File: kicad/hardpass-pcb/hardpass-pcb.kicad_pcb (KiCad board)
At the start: 2 copper layers, 30 x 65 mm, 37 parts, among them P1 Pi_Zero, P2 OLED_I2C, SW1 1, SW10 C/UP, SW11 0/OK, SW12 OK/DN, SW2 2, SW3 3, SW4 4, SW5 5, SW6 6, SW7 7, SW8 8, SW9 9, U2 ESP-12E

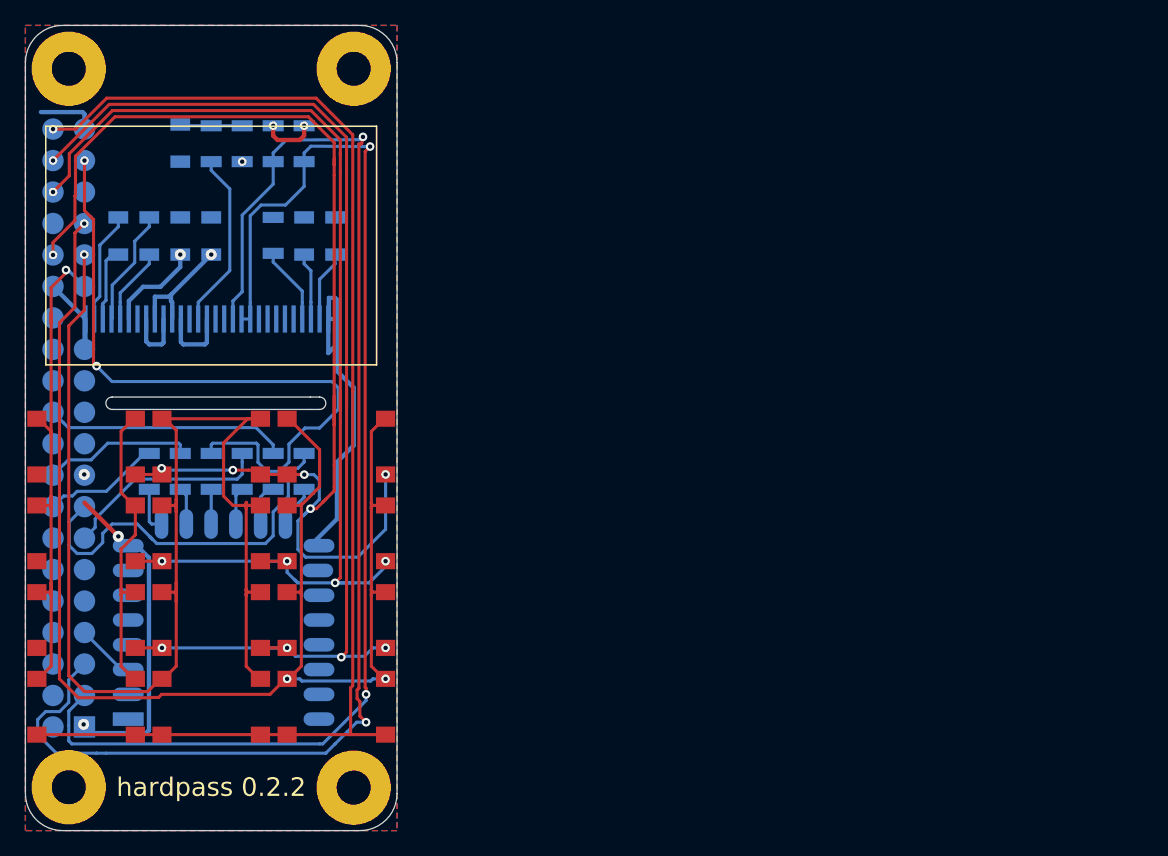
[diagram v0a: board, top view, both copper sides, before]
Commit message: routed 2nd board
not finished, but a start
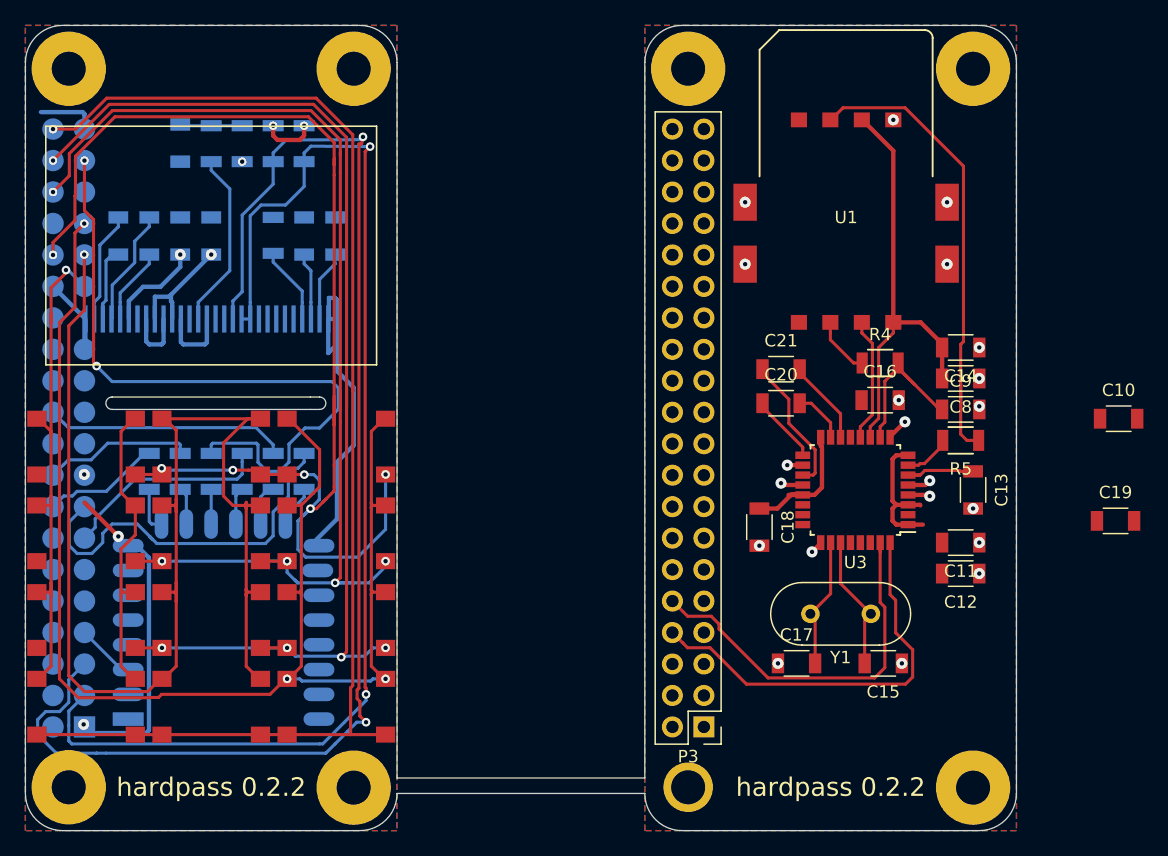
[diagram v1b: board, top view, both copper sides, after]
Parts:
- added C10: 100pF, Capacitors_SMD:C_1206, F.Cu at (88.2, 31.8)
- added C11: 10µF, Capacitors_SMD:C_1206, F.Cu at (75.5, 41.8)
- added C12: 100nF, Capacitors_SMD:C_1206, F.Cu at (75.5, 44.2)
- added C13: 22nF, Capacitors_SMD:C_1206, F.Cu at (76.5, 37.5)
- added C14: 100pF, Capacitors_SMD:C_1206, F.Cu at (75.5, 26.0)
- added C15: 22pF, Capacitors_SMD:C_1206, F.Cu at (69.2, 51.5)
- added C16: 220nF, Capacitors_SMD:C_1206, F.Cu at (69.0, 30.2)
- added C17: 22pF, Capacitors_SMD:C_1206, F.Cu at (62.2, 51.5)
- added C18: 100nF, Capacitors_SMD:C_1206, F.Cu at (59.2, 40.5)
- added C19: 10µF, Capacitors_SMD:C_1206, F.Cu at (88.0, 40.0)
- added C20: 220nF, Capacitors_SMD:C_1206, F.Cu at (61.0, 30.5)
- added C21: 220nF, Capacitors_SMD:C_1206, F.Cu at (61.0, 27.8)
- added C8: 220nF, Capacitors_SMD:C_1206, F.Cu at (75.5, 28.5)
- added C9: 33pF, Capacitors_SMD:C_1206, F.Cu at (75.5, 31.0)
- added P3: Pi_Zero, hardpass:Pin_Header_Straight_2x20_Pitch2.54mm_centered, F.Cu at (53.5, 32.5)
- added R4: 100, Resistors_SMD:R_1206, F.Cu at (69.0, 27.2)
- added R5: 180, Resistors_SMD:R_1206, F.Cu at (75.5, 33.5)
- added REF**: 1pin, hardpass:1pin_nosilk, F.Cu at (76.5, 61.5)
- added REF**: 1pin, hardpass:1pin_nosilk, F.Cu at (76.5, 3.50)
- added REF**: 1pin, hardpass:1pin_nosilk, F.Cu at (53.5, 3.50)
- added REF**: 1pin, hardpass:1pin_nosilk, F.Cu at (53.5, 61.5)
- added U1: ISO7816, hardpass:CAF99-08153-S132, F.Cu at (66.2, 16.0)
- added U3: TDA8029, Housings_QFP:LQFP-32_7x7mm_Pitch0.8mm, F.Cu at (67.0, 37.5)
- added Y1: 14.745MHz, Crystals:Crystal_HC49-U_Vertical, F.Cu at (68.2, 47.5)
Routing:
- net Net-(R5-Pad1): track 0.00 -> 38.5 mm
- net Net-(C14-Pad2): track 0.00 -> 34.9 mm
- net CARD_RX: track 0.00 -> 33.0 mm
- net CARD_TX: track 0.00 -> 31.3 mm
- net +5V: track 0.00 -> 23.3 mm
- net Net-(C9-Pad1): track 0.00 -> 13.3 mm
- net Net-(C21-Pad1): track 0.00 -> 11.2 mm
- net Net-(C15-Pad2): track 0.00 -> 11.0 mm
- net Net-(C17-Pad2): track 0.00 -> 10.6 mm
- net Net-(C10-Pad2): track 0.00 -> 10.0 mm
- net GND: track 52.9 -> 62.5 mm, vias 0 -> 17
- net Net-(C21-Pad2): track 0.00 -> 6.87 mm
- net Net-(C13-Pad1): track 0.00 -> 6.29 mm
- net Net-(C20-Pad1): track 0.00 -> 5.55 mm
- net Net-(R4-Pad1): track 0.00 -> 4.75 mm
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- added copper zone on F.Cu, net +5V
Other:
- board size 30 x 65 mm -> 80 x 65 mm
